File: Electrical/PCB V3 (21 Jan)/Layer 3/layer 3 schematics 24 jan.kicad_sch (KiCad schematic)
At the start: 22 parts, among them J1 Conn_01x06, J2 Conn_01x02, J3 Conn_01x06, J4 Conn_01x06, J5 Conn_01x06, J7 Conn_01x08, J8 Conn_01x02, U2 XT30UPB-M, U3 4754

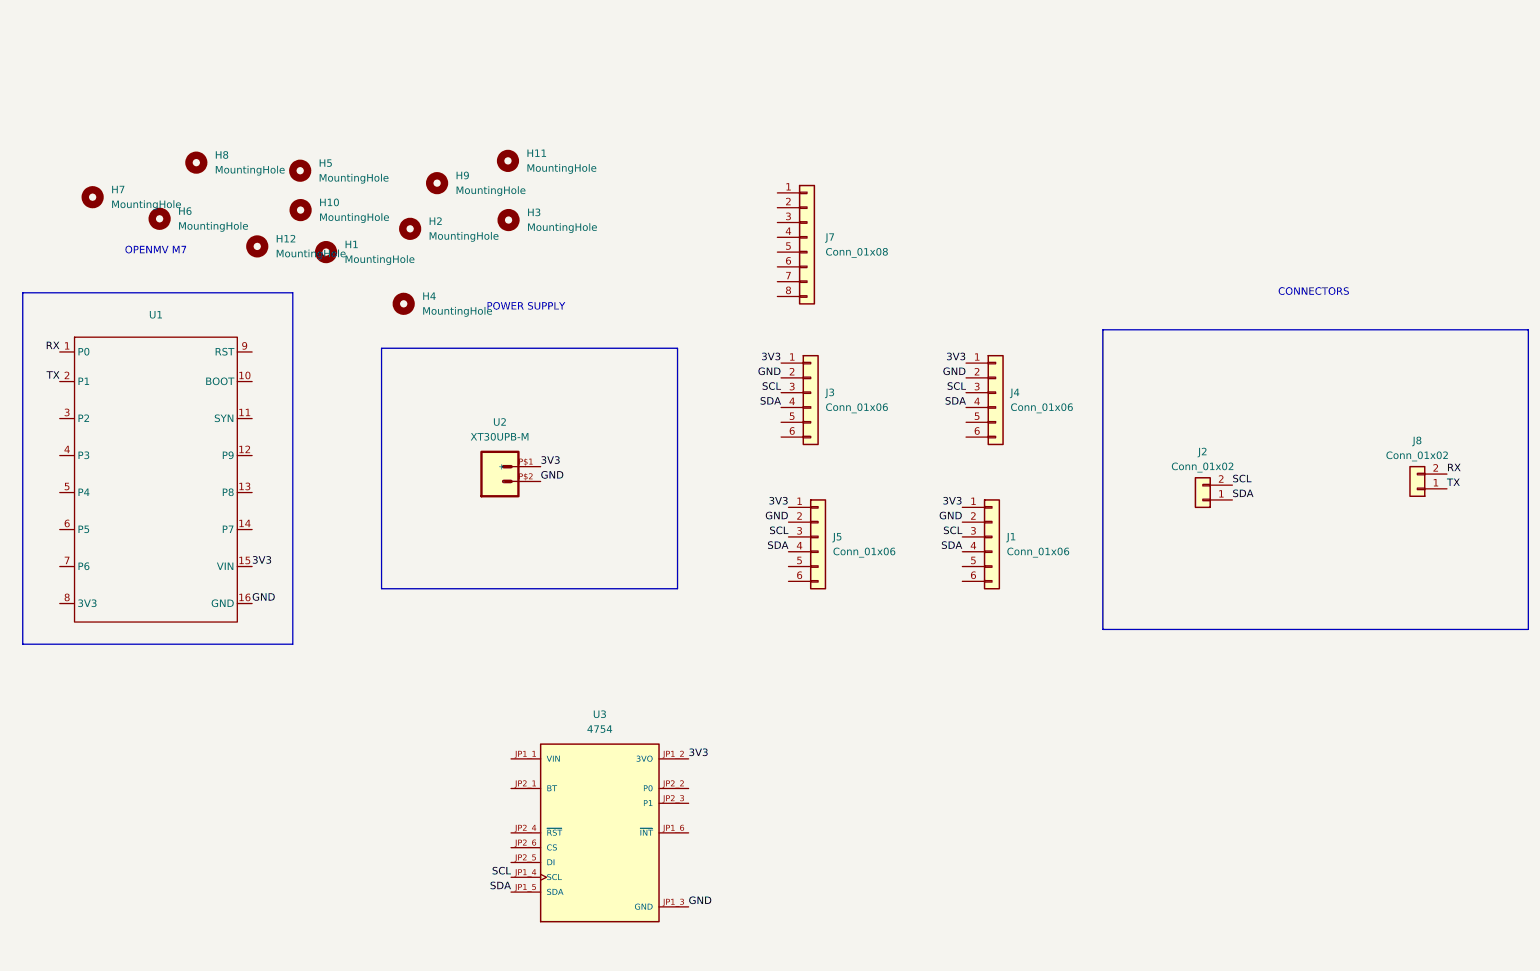
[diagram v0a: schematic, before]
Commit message: 7 feb update!!! stop at pull up res
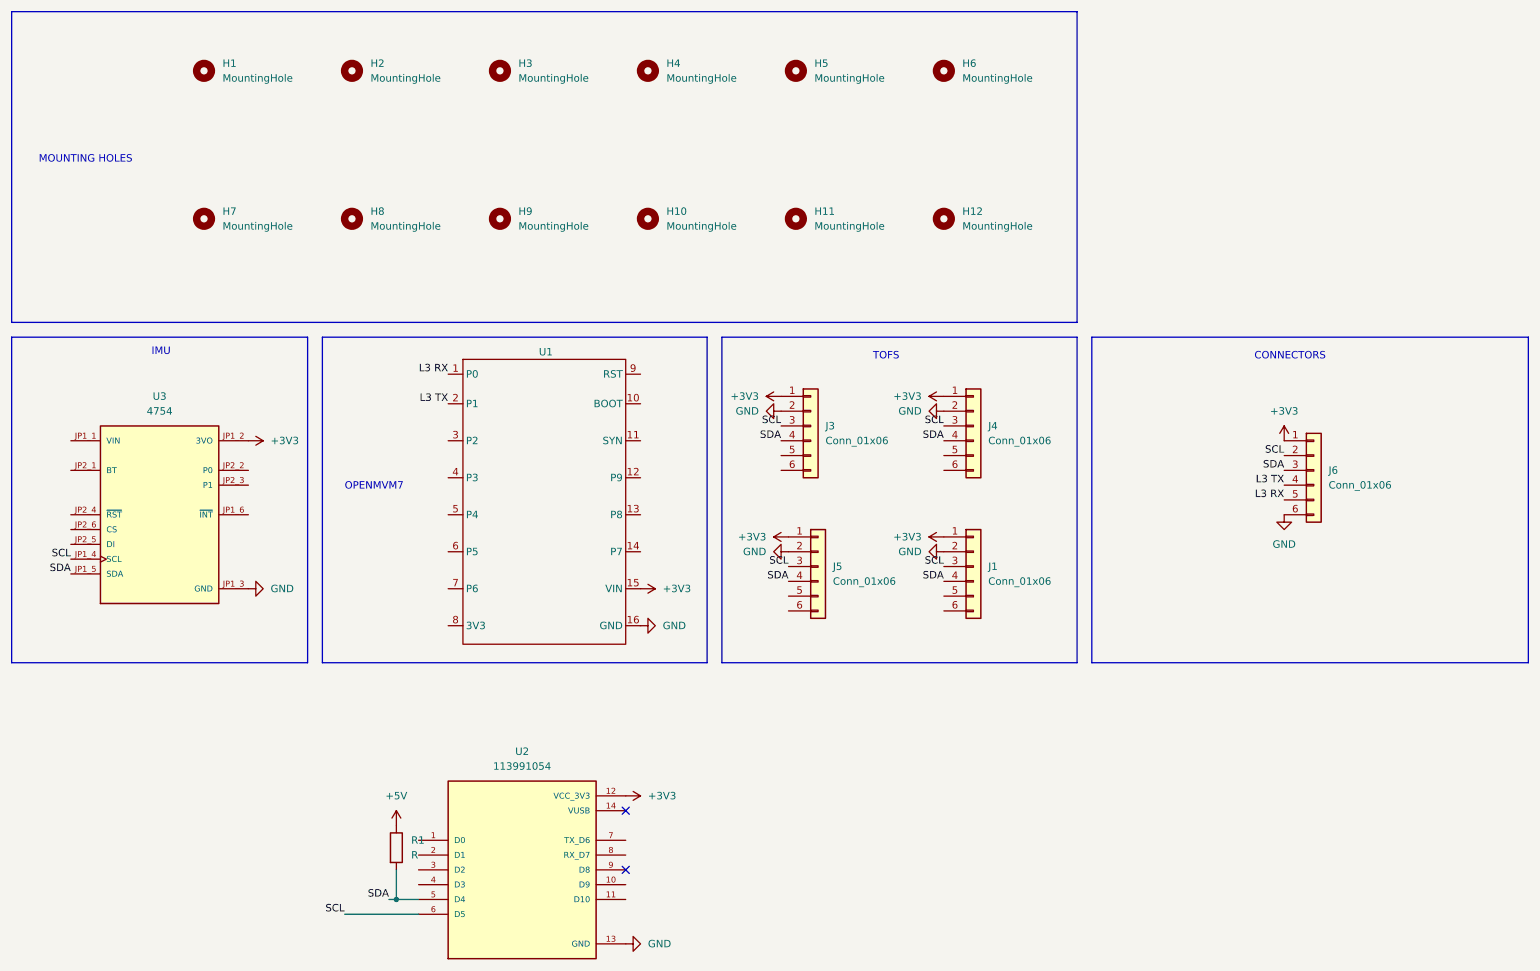
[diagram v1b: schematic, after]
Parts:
- removed J2, J8: Conn_01x02, Connector_PinHeader_1.00mm:PinHeader_1x02_P1.00mm_Vertical, symbol Connector_Generic:Conn_01x02
- removed J7: Conn_01x08, Connector_PinHeader_1.00mm:PinHeader_1x08_P1.00mm_Vertical, symbol Connector_Generic:Conn_01x08
- removed U2: XT30UPB-M, XT30UPB-M:XT30UPB-M, symbol XT30UPB-M:XT30UPB-M
- added J6: Conn_01x06, Connector_JST:JST_EH_B6B-EH-A_1x06_P2.50mm_Vertical, symbol Connector_Generic:Conn_01x06
- added R1: R, symbol Device:R
- added U2: 113991054, Layer1_Symbol_Footprints:XiaoSeeedStudioEsp32, symbol XiaoSeeedStudioEsp32:113991054
- H1, H10, H11, H12, H2, H3, H4, H5, H6, H7, H8, H9: footprint MountingHole:MountingHole_3.2mm_M3 -> MountingHole:MountingHole_3.2mm_M3_Pad_Via
- J1, J3, J4, J5: footprint Connector_PinHeader_1.00mm:PinHeader_1x06_P1.00mm_Vertical -> Connector_PinHeader_2.54mm:PinHeader_1x06_P2.54mm_Vertical
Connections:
- net GND: now also J6.6 (Pin_6), U2.13 (GND)
- net SCL: now also J6.2 (Pin_2), U2.6 (D5)
- net SDA: now also J6.3 (Pin_3), R1.2, U2.5 (D4)
- net 3V3 renamed +3V3
- net +3V3: now also J6.1 (Pin_1), U2.12 (VCC_3V3)
- net RX renamed L3 RX
- net L3 RX: now also J6.5 (Pin_5)
- net TX renamed L3 TX
- net L3 TX: now also J6.4 (Pin_4)
- new net +5V: R1.1
- no-connect marks 0 -> 2
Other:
- note added: "IMU"
- note added: "MOUNTING HOLES"
- note added: "OPENMVM7"
- note added: "TOFS"
- note removed: "OPENMV M7"
- note removed: "POWER SUPPLY"
- moved on the sheet: H1, H10, H11, H12, H2, H3, H4, H5, H6, H7, H8, H9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
